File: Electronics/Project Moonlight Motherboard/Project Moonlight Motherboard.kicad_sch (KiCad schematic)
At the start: 42 parts, among them M1 AO3400A, M2 AO3400A, M3 AO3400A, U1 STM32F407IEHx, U2 TMC2209_SILENTSTEPSTICK, U3 TMC2209_SILENTSTEPSTICK, U4 TMC2209_SILENTSTEPSTICK, U5 TMC2209_SILENTSTEPSTICK

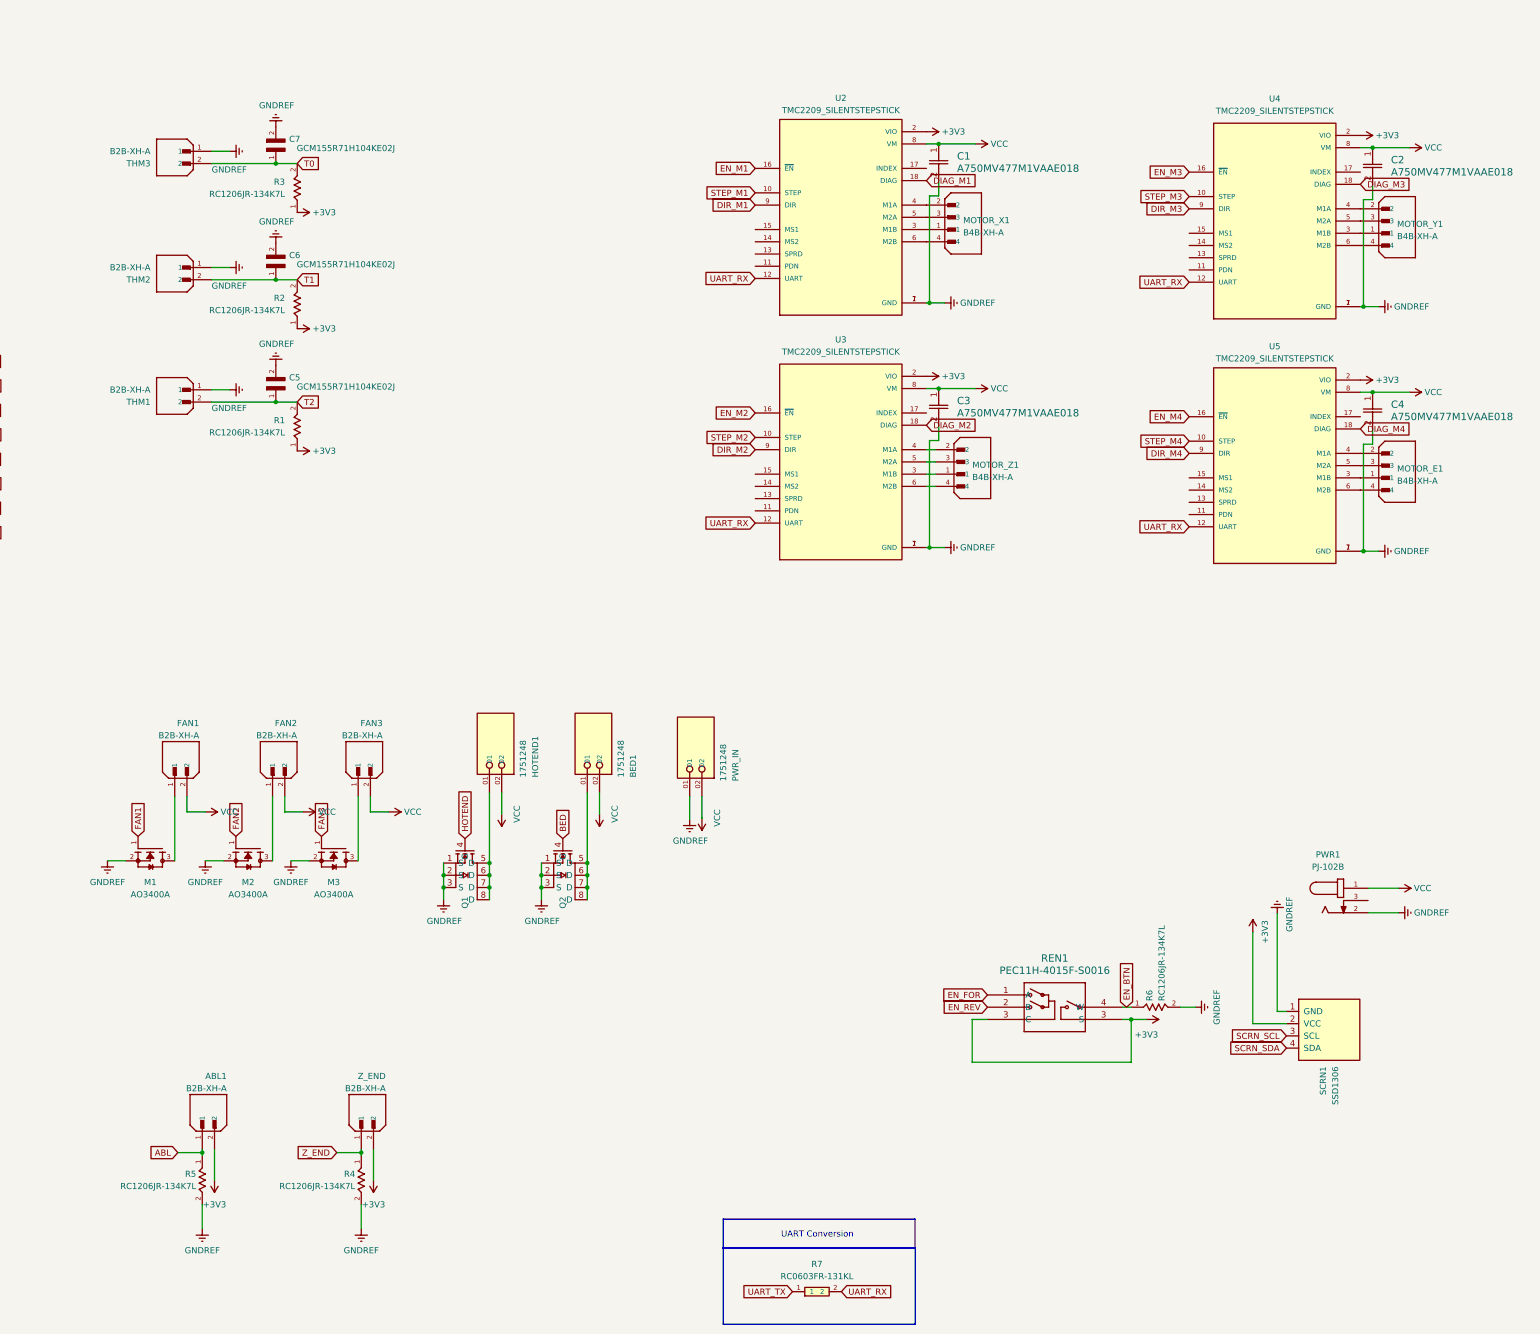
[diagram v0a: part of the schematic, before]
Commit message: whoops forgor to save it
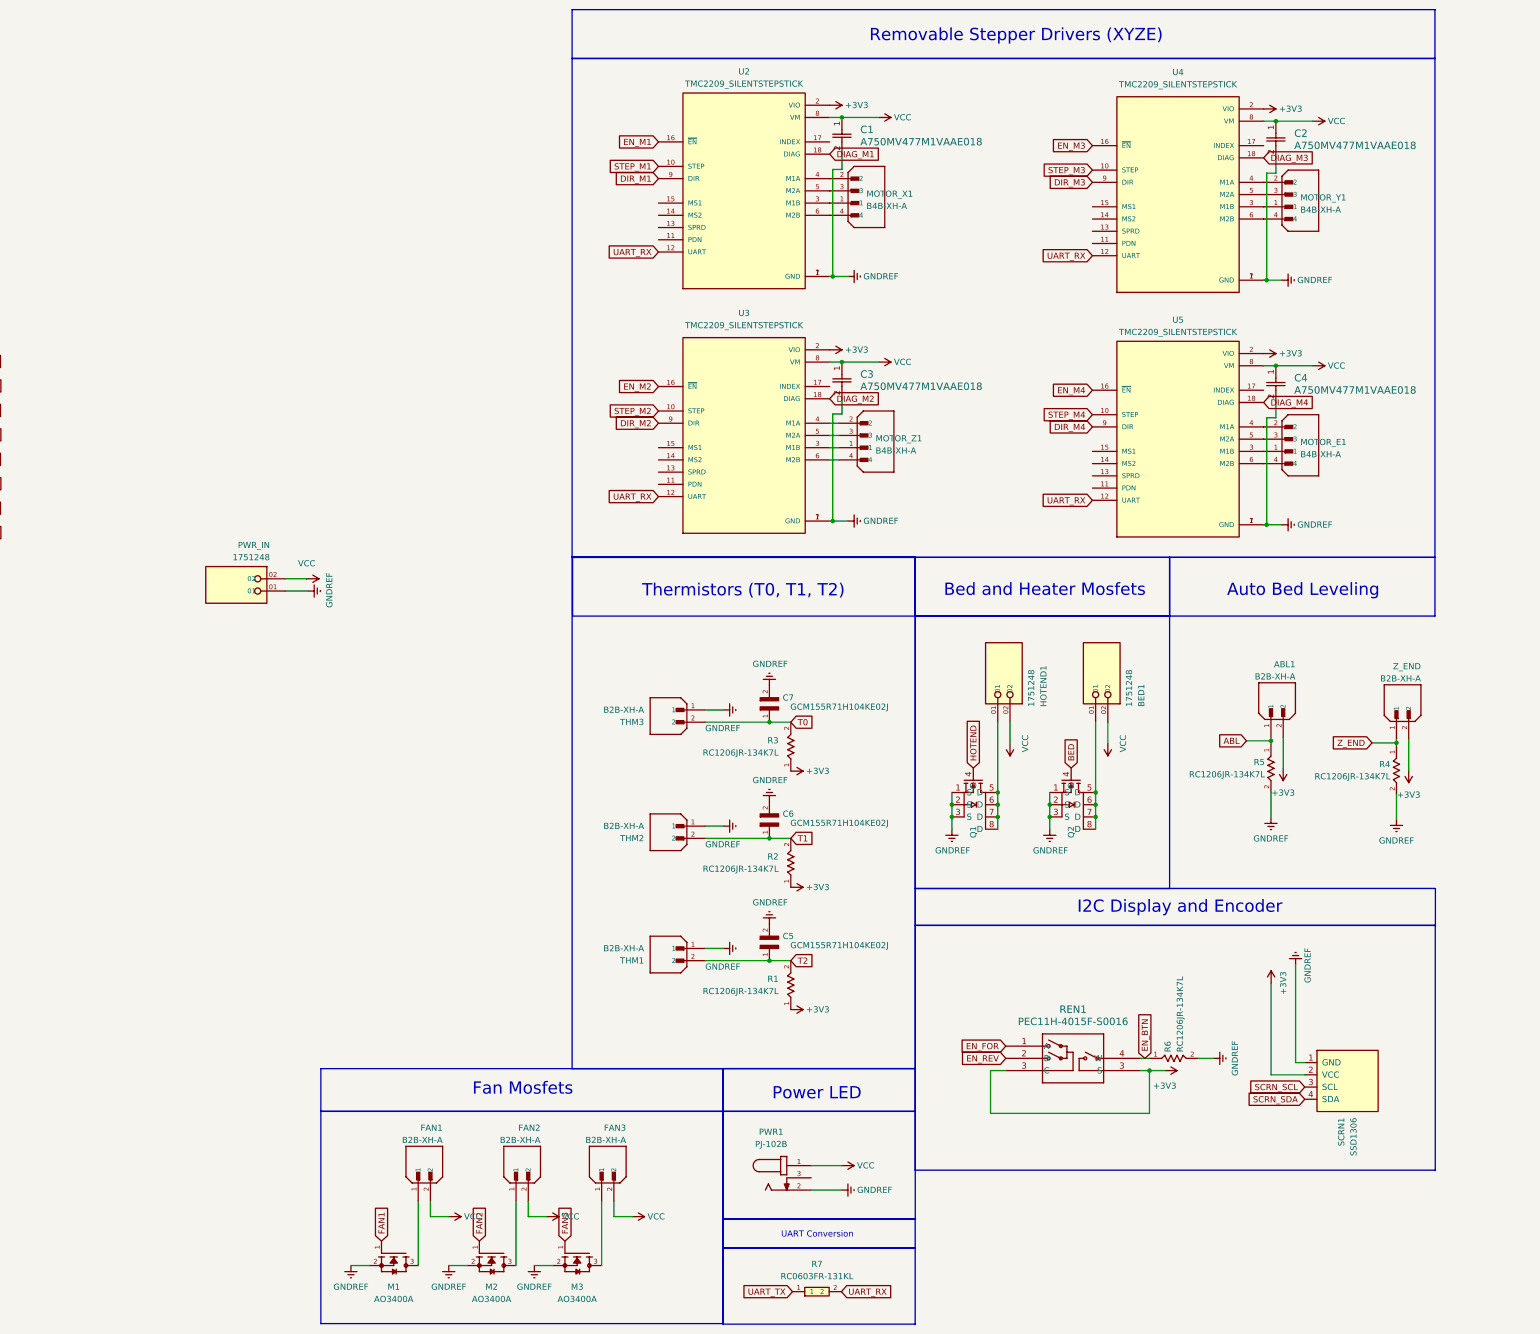
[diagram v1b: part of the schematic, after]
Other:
- note added: "Auto Bed Leveling"
- note added: "Bed and Heater Mosfets"
- note added: "Fan Mosfets"
- note added: "I2C Display and Encoder"
- note added: "Power LED"
- note added: "Removable Stepper Drivers (XYZE)"
- note added: "Thermistors (T0, T1, T2)"
- moved on the sheet: ABL1, BED1, C1, C2, C3, C4, C5, C6, C7, FAN1, FAN2, FAN3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
